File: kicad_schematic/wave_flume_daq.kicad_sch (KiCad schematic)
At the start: 39 parts, among them J1 M12 B-5, J2 M12 B-5, J3 M12 B-5, J4 M12 B-5, J5 M12 A-5, J6 M12 A-5, J7 M12 A-5, J8 M12 A-5, J9 C14 inlet, U1 IAA100 (at flume), U2 IAA100 (at flume), U3 IAA100 (at flume)

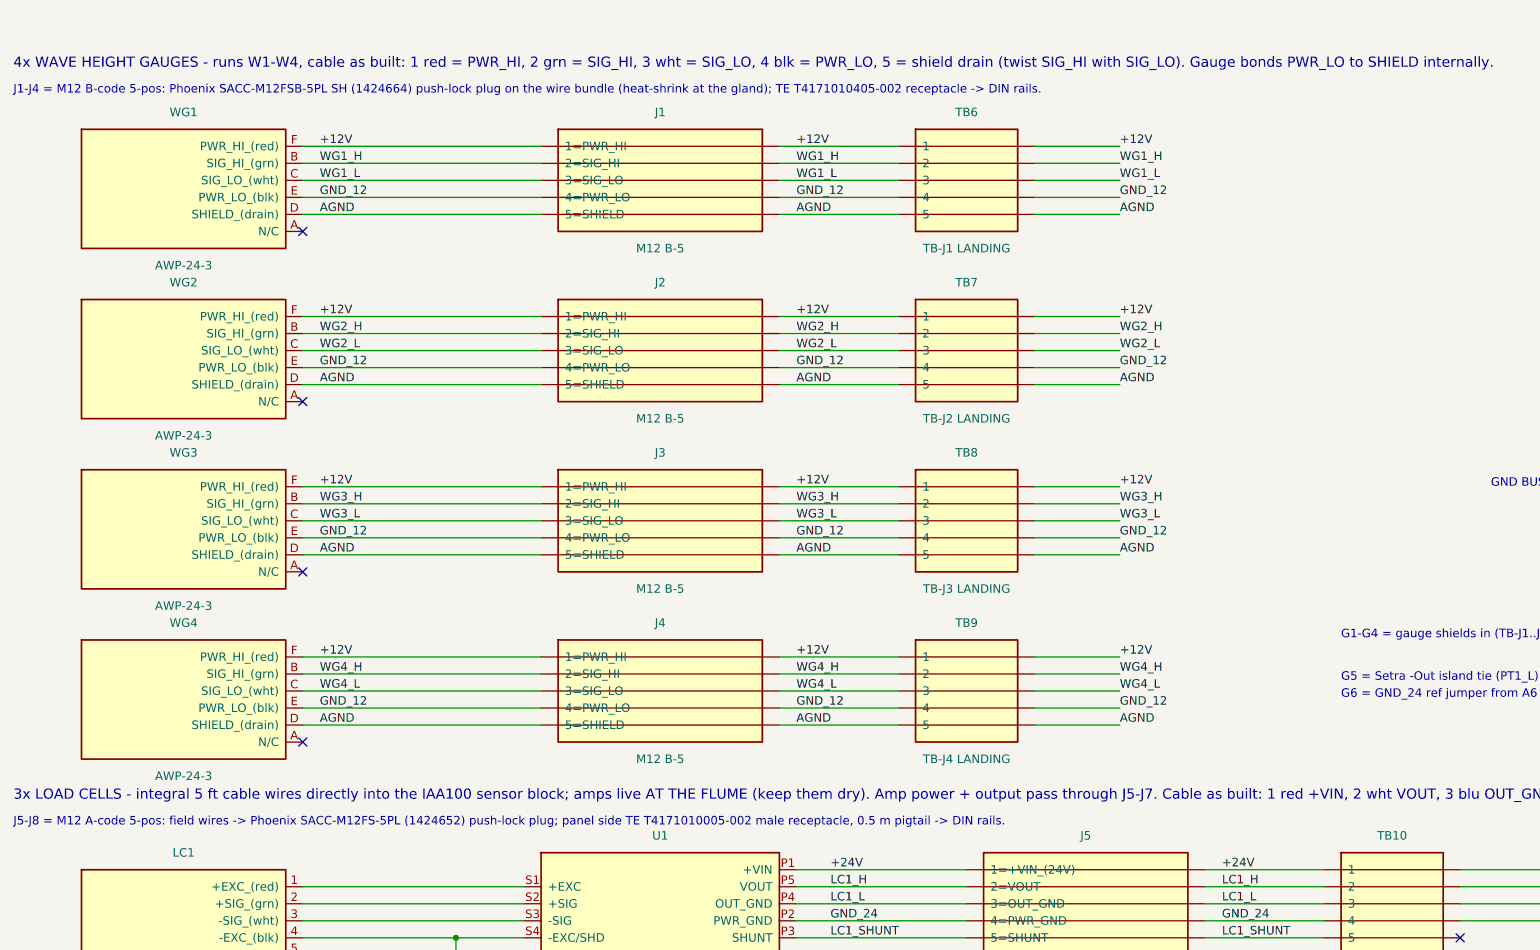
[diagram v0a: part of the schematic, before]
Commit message: clean up text in docs
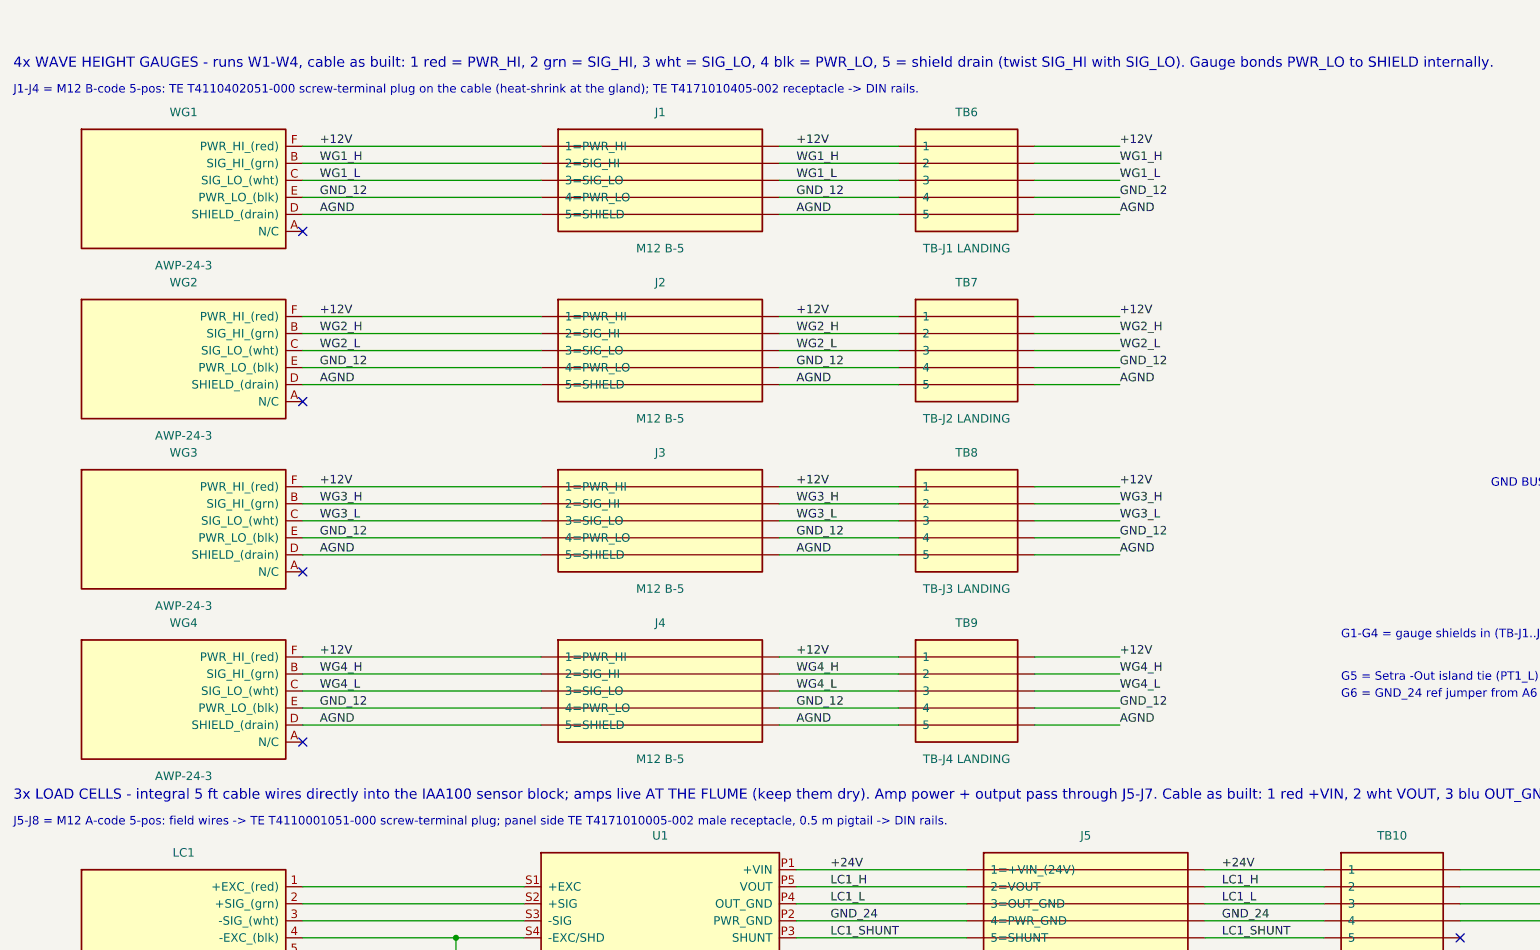
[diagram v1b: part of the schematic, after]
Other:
- note added: "J1-J4 = M12 B-code 5-pos: TE T4110402051-000 screw-terminal plug on the cable (heat-shrink at the gland); TE T4171010405-002 receptacle -> DIN rails."
- note added: "J5-J8 = M12 A-code 5-pos: field wires -> TE T4110001051-000 screw-terminal plug; panel side TE T4171010005-002 male receptacle, 0.5 m pigtail -> DIN rails."
- note removed: "J1-J4 = M12 B-code 5-pos: Phoenix SACC-M12FSB-5PL SH (1424664) push-lock plug on the wire bundle (heat-shrink at the gland); TE T4171010405-002 receptacle -> DIN rails."
- note removed: "J5-J8 = M12 A-code 5-pos: field wires -> Phoenix SACC-M12FS-5PL (1424652) push-lock plug; panel side TE T4171010005-002 male receptacle, 0.5 m pigtail -> DIN rails."
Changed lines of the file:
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@@
 		)
 	)
-	(text "J5-J8 = M12 A-code 5-pos: field wires -> Phoenix SACC-M12FS-5PL (1424652) push-lock plug; panel side TE T4171010005-002 male receptacle, 0.5 m pigtail -> DIN rails."
+	(text "J5-J8 = M12 A-code 5-pos: field wires -> TE T4110001051-000 screw-terminal plug; panel side TE T4171010005-002 male receptacle, 0.5 m pigtail -> DIN rails."
 		(exclude_from_sim no)
 		(at 30.48 146.05 0)
@@
 		)
 	)
-	(text "J1-J4 = M12 B-code 5-pos: Phoenix SACC-M12FSB-5PL SH (1424664) push-lock plug on the wire bundle (heat-shrink at the gland); TE T4171010405-002 receptacle -> DIN rails."
+	(text "J1-J4 = M12 B-code 5-pos: TE T4110402051-000 screw-terminal plug on the cable (heat-shrink at the gland); TE T4171010405-002 receptacle -> DIN rails."
 		(exclude_from_sim no)
 		(at 30.48 36.83 0)
